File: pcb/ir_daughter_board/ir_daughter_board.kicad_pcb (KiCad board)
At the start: 2 copper layers, 60 x 36 mm, 43 parts, among them IC1 TS2596SCS, J1 USB_OTG, J2 Conn_01x06, J3 Conn_01x06, SW1 BOOT, SW2 RESET, U1 MCP2200T-I/SS, U3 ESP-WROOM-02, Y1 12,0000-HC49-SMD

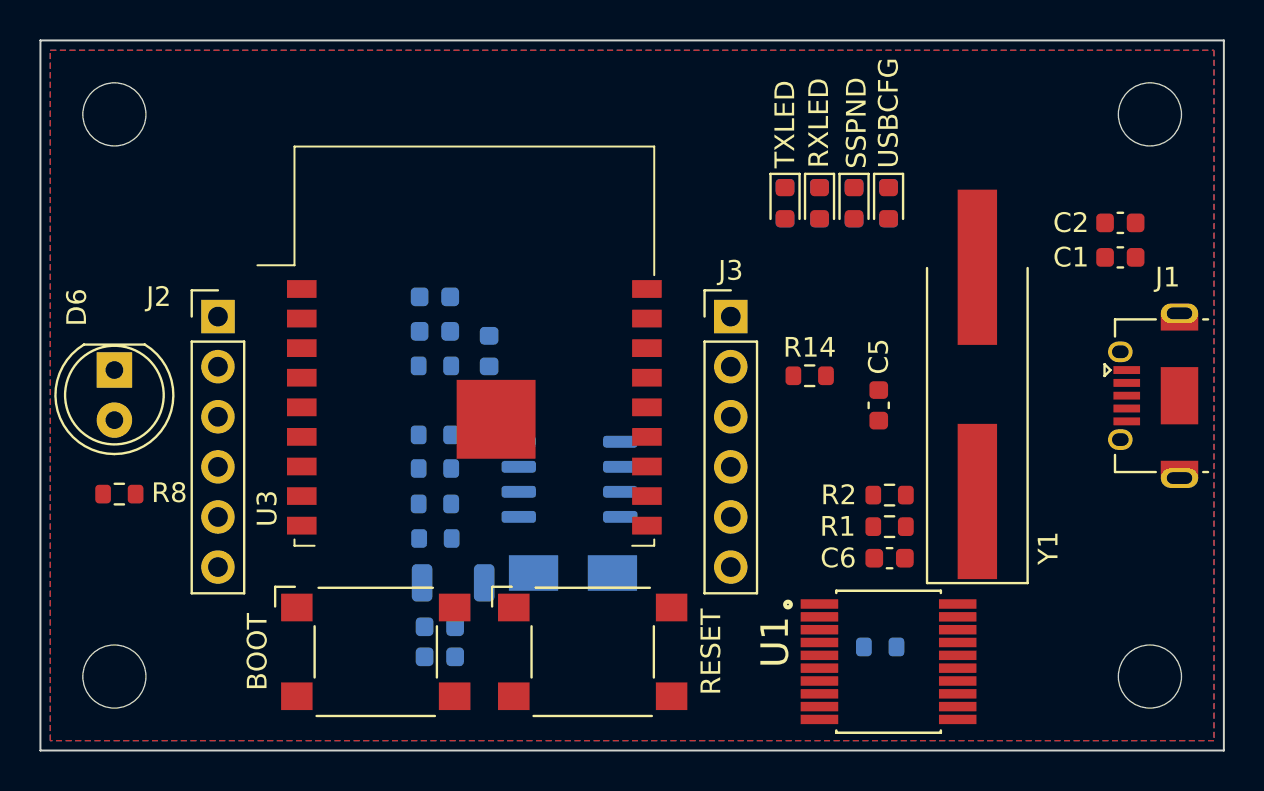
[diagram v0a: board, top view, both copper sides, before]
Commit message: updated schematic
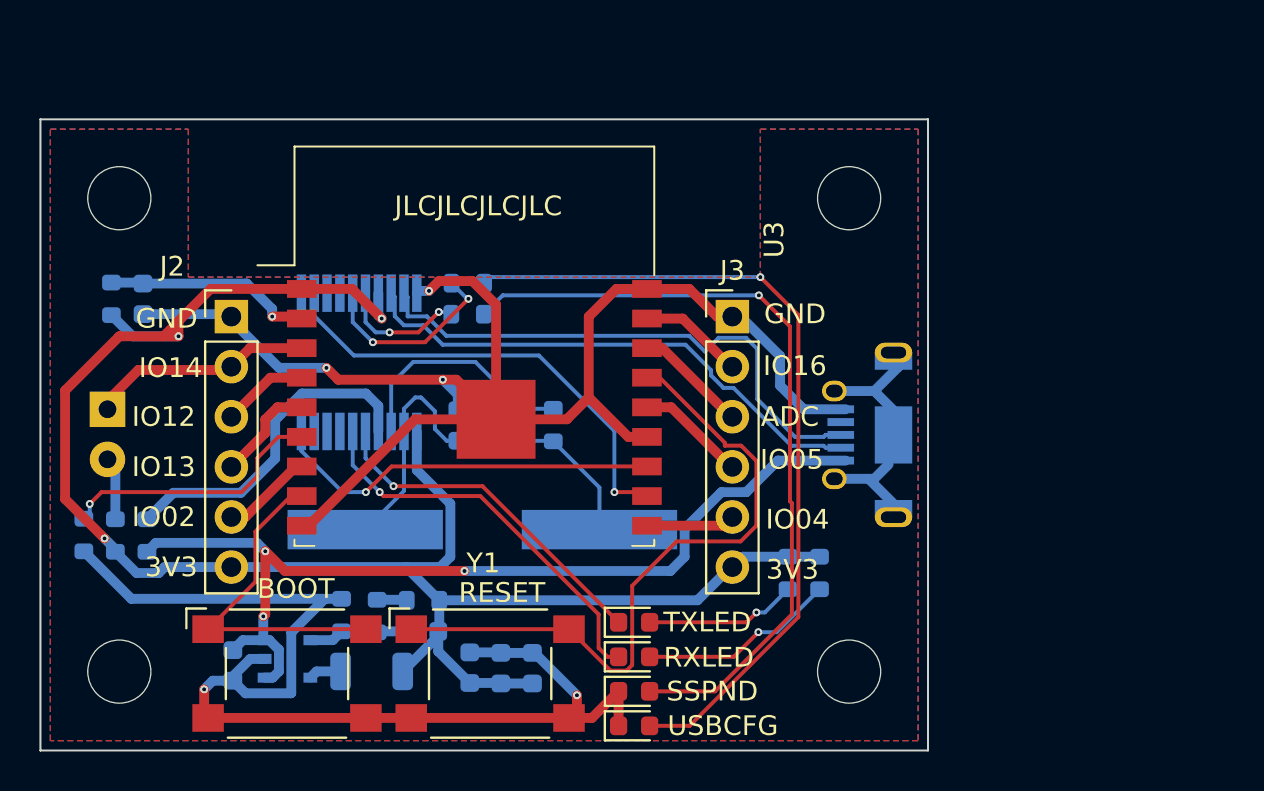
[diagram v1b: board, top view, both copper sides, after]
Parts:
- removed C3: 470uF, Capacitor_SMD:C_0603_1608Metric
- removed D1: SK34A, Diode_SMD:D_SMA
- removed R12: 1k5, Resistor_SMD:R_0603_1608Metric
- C1: value 4.7uF -> 10uF; moved to B.Cu
- C2: value 0.1uF -> 18pF; moved to B.Cu
- C4: value 0.1uF -> 10uF
- C5, C6, D6, J1, R1, R14, R2, R8, U1, Y1: moved to B.Cu
- IC1: value TS2596SCS -> NCP1521BSN; footprint Package_SO:SO-8_3.9x4.9mm_P1.27mm -> Package_SO:TSOP-5_1.65x3.05mm_P0.95mm
- L1: value 33uH -> 2.2uH
- R10: value 100k -> 1k
- R11: value 1k -> 4k3
- R13: value 1k5 -> 200R
- moved C1 49.5 mm to (106.8, 108.7), turned to -90 degrees
- moved C2 41.0 mm to (116.4, 107.0)
- moved R14 37.7 mm to (99.2, 102.1), turned to 90 degrees
- moved R3 37.6 mm to (102.4, 102.1), turned to 90 degrees
- moved U1 30.8 mm to (113.2, 93.3), turned to 90 degrees
- moved D4 29.5 mm to (127.1, 111.8), turned to 0 degrees
- moved D5 27.1 mm to (127.1, 110.0), turned to 0 degrees
- moved Y1 26.2 mm to (119.4, 101.8), turned to 180 degrees
- moved D3 24.8 mm to (127.1, 108.2), turned to 0 degrees
- moved D2 22.6 mm to (127.1, 106.5), turned to 0 degrees
- moved R6 21.7 mm to (118.7, 89.3), turned to 0 degrees
- moved C5 21.4 mm to (118.2, 96.5)
- moved C6 21.3 mm to (119.8, 96.5), turned to -90 degrees
- moved R7 20.4 mm to (118.7, 90.9), turned to 180 degrees
- moved R1 19.4 mm to (121.4, 96.5), turned to -90 degrees
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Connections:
- C2 pad 1: +5V -> +3V3
- C2 pad 2: GND -> Net-(C2-Pad2)
- D4 pad 1: USBCFG -> GND
- D5 pad 1: SSPND -> GND
- D6 pad 1: GND -> IR
- D6 pad 2: IR -> Net-(D6-Pad2)
- IC1 pad 2: Net-(D1-Pad1) -> GND
- IC1 pad 3: Net-(IC1-Pad3) -> +5V
- IC1 pad 4: Net-(IC1-Pad4) -> Net-(C2-Pad2)
- IC1 pad 5: GND -> Net-(IC1-Pad5)
- J2 pad 2: GPIO 05 -> IR
- J2 pad 3: GPIO 04 -> GPIO 12
- J2 pad 4: GPIO 02 -> GPIO 13
- J2 pad 5: ADC -> GPIO 02
- J3 pad 2: IR -> GPIO 16
- J3 pad 3: GPIO 16 -> ADC
- J3 pad 4: GPIO 13 -> GPIO 05
- J3 pad 5: GPIO 12 -> GPIO 04
- L1 pad 1: Net-(D1-Pad1) -> Net-(IC1-Pad5)
- R10 pad 1: Net-(IC1-Pad4) -> Net-(C2-Pad2)
- R13 pad 2: Net-(IC1-Pad3) -> Net-(C2-Pad2)
- R6 pad 1: +3V3 -> USBCFG
- R7 pad 2: +3V3 -> SSPND
- R8 pad 1: IR -> Net-(D6-Pad2)
- U1 pad 11: unconnected-(U1-Pad11) -> /USB_to_UART/RTS
- U1 pad 13: unconnected-(U1-Pad13) -> /USB_to_UART/CTS
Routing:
- net GND: track 0.00 -> 133.2 mm, vias 0 -> 5
- net +3V3: track 0.00 -> 92.5 mm, vias 0 -> 3
- net +5V: track 0.00 -> 48.6 mm, vias 0 -> 3
- net Net-(D4-Pad2): track 0.00 -> 42.0 mm, vias 0 -> 1
- net Net-(D5-Pad2): track 0.00 -> 40.0 mm, vias 0 -> 1
- net Net-(SW2-Pad1): track 0.00 -> 33.8 mm
- net /USB_to_UART/USB_D+: track 0.00 -> 28.1 mm
- net /USB_to_UART/USB_D-: track 0.00 -> 27.0 mm
- net /IR_Remote_Circuit/TXD: track 0.00 -> 23.3 mm, vias 0 -> 1
- net RXLED: track 0.00 -> 20.2 mm, vias 0 -> 1
- net /IR_Remote_Circuit/RXD: track 0.00 -> 19.9 mm, vias 0 -> 1
- net TXLED: track 0.00 -> 17.6 mm, vias 0 -> 1
- net Net-(R3-Pad2): track 0.00 -> 17.1 mm
- net Net-(SW1-Pad1): track 0.00 -> 16.5 mm
- net Net-(R14-Pad2): track 0.00 -> 13.6 mm, vias 0 -> 1
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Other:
- board size 60 x 36 mm -> 45 x 32 mm
